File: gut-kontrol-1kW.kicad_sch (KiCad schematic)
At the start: 3 parts

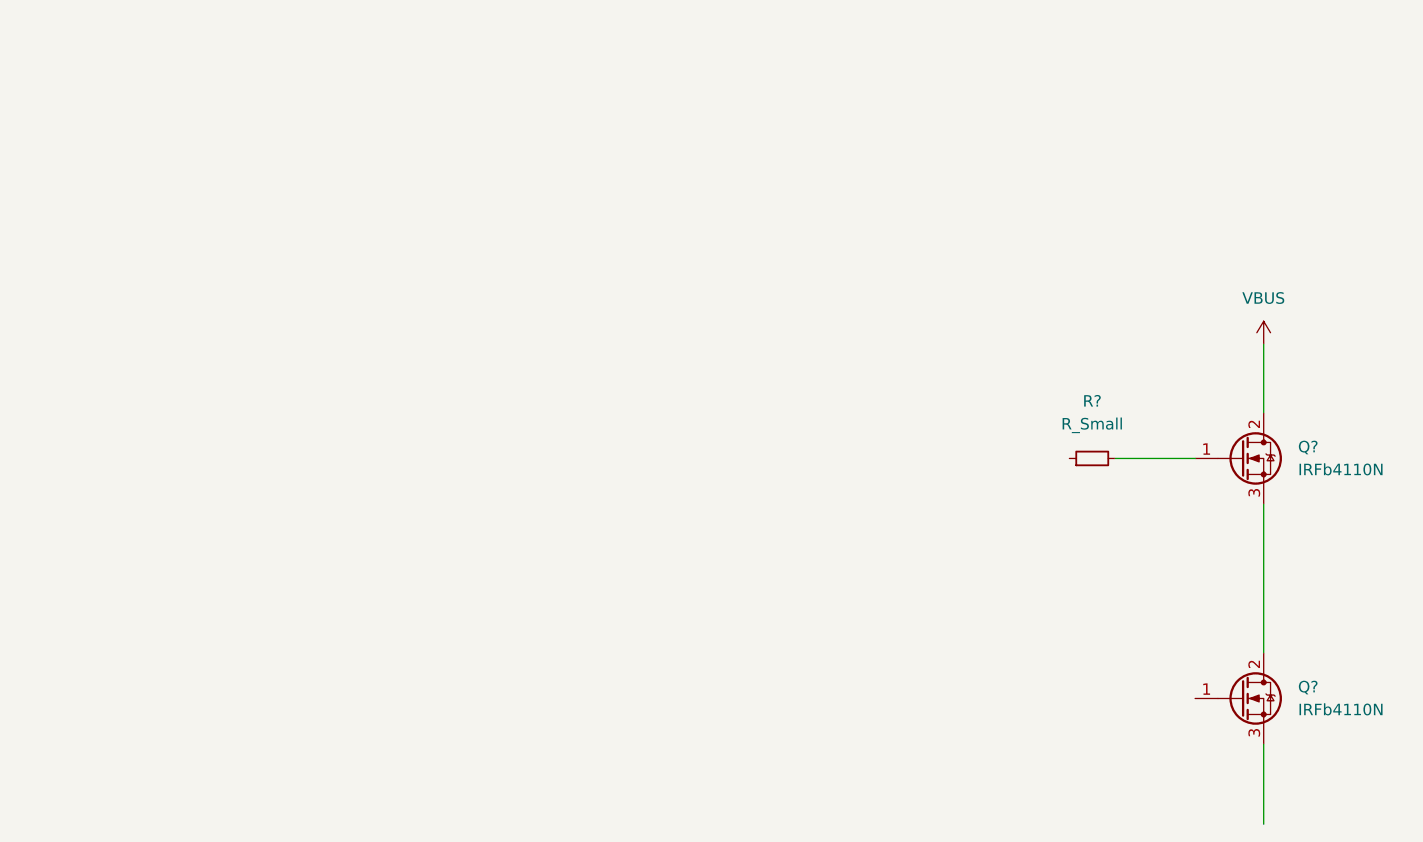
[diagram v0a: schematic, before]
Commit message: Done with the powerstage
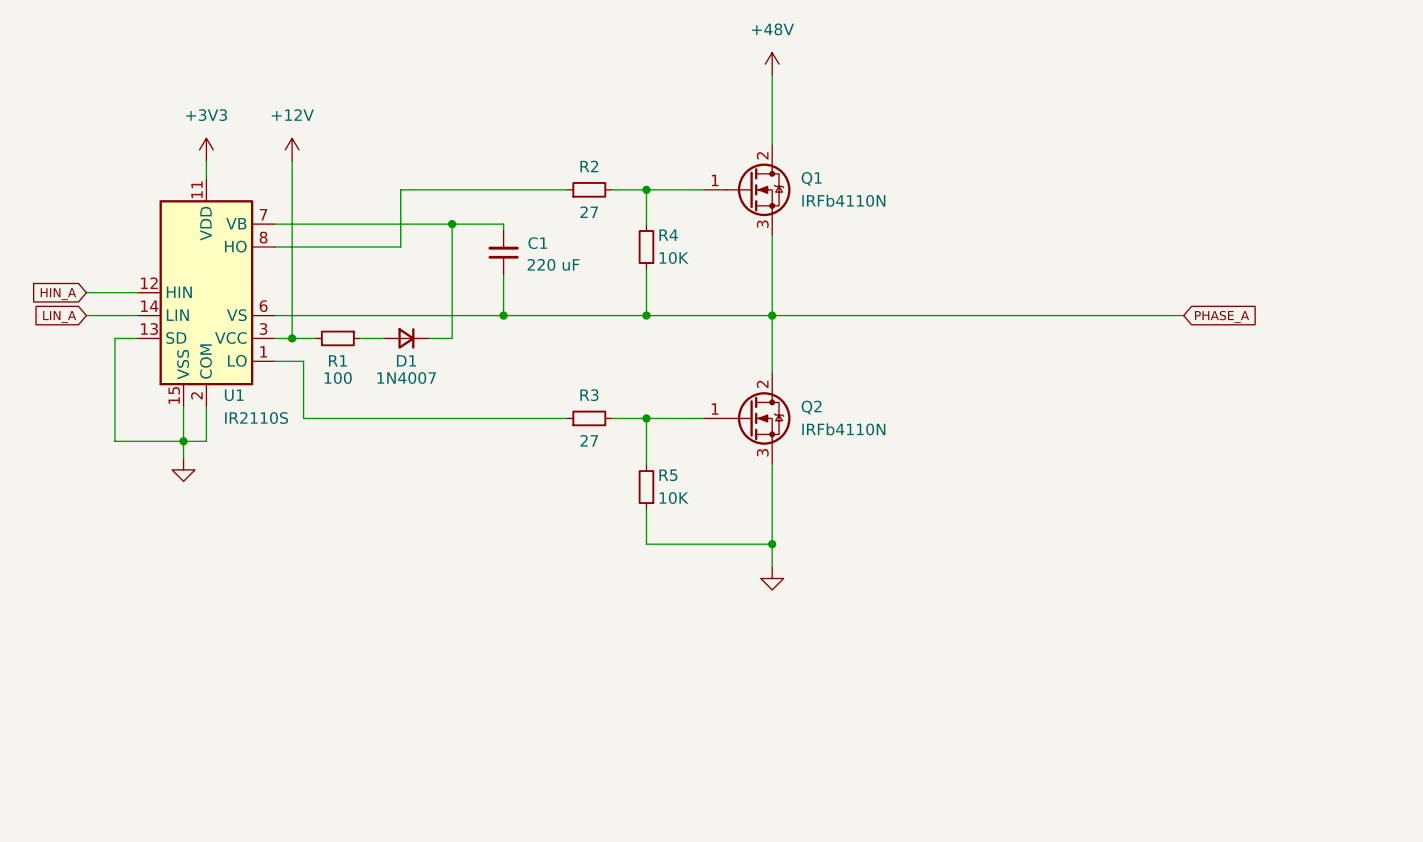
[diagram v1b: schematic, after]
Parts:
- added C1: 220 uF, Capacitor_SMD:C_0805_2012Metric_Pad1.18x1.45mm_HandSolder, symbol Device:C_Small
- added D1: 1N4007, Diode_SMD:D_SMA-SMB_Universal_Handsoldering, symbol Device:D_Small
- added R1: 100, Resistor_SMD:R_0805_2012Metric_Pad1.20x1.40mm_HandSolder, symbol Device:R_Small
- added R3: 27, Resistor_SMD:R_0805_2012Metric_Pad1.20x1.40mm_HandSolder, symbol Device:R_Small
- added R4, R5: 10K, Resistor_SMD:R_0805_2012Metric_Pad1.20x1.40mm_HandSolder, symbol Device:R_Small
- added U1: IR2110S, Package_SO:SOIC-16W_7.5x10.3mm_P1.27mm, symbol Driver_FET:IR2110S
- R2: renamed from R?; value R_Small -> 27; footprint (none) -> Resistor_SMD:R_0805_2012Metric_Pad1.20x1.40mm_HandSolder
- gave numbers to parts that had none: 2
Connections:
- net at Q1.1 (G), R2.2: now also R4.2
- net PHASE_A: now reaches Q1.3 (S), Q2.2 (D)
- net PHASE_A: now also C1.1, R4.1, U1.6 (VS)
- net at R2.1: now also U1.8 (HO)
- net at Q2.1 (G): now also R3.2, R5.2
- net GND: now reaches Q2.3 (S)
- net GND: now also R5.1, U1.13 (SD), U1.15 (VSS), U1.2 (COM)
- net VBUS renamed +48V
- new net: C1.2, D1.1 (K), U1.7 (VB)
- new net: R3.1, U1.1 (LO)
- new net: D1.2 (A), R1.1
- new net +12V: R1.2, U1.3 (VCC)
- new net +3V3: U1.11 (VDD)
- new net HIN_A: U1.12 (HIN)
- new net LIN_A: U1.14 (LIN)
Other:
- moved on the sheet: Q1, Q2, R2
